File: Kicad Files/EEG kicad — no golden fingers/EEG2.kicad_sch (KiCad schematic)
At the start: 263 parts, among them J1 Conn_01x05_Pin, J2 Conn_01x11_Pin, U1 AD5293, U10 LF356N, U11 LF356N, U12 LF356N, U123 LF356N, U124 AD5293, U125 AD5293, U126 AD5293, U127 AD5293, U128 AD5293, U13 LF356N, U14 AD5293, U15 INA823, U16 INA823, U17 LF356N, U18 LF356N, U19 LF356N, U2 INA823, U20 LF356N, U21 LF356N, U22 LF356N, U23 LF356N, U24 LF356N, U25 AD5293, U26 AD5293, U27 INA823, U28 LF356N, U29 LF356N, U3 LF356N, U30 LF356N, U31 LF356N, U32 AD5293, U4 LF356N, U5 LF356N, U6 LF356N, U7 Teensy4.1, U75 INA823, U76 INA823, U77 INA823, U78 INA823, U79 INA823, U80 LF356N, U81 LF356N, U82 LF356N, U83 LF356N, U84 LF356N, U85 LF356N, U86 LF356N, U87 LF356N, U88 LF356N, U89 LF356N, U9 INA823, U90 LF356N, U91 LF356N, U92 LF356N, U93 LF356N, U94 LF356N, U95 LF356N, U96 LF356N, U97 LF356N, U98 LF356N

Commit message: Corrections in EEG
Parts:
- removed C101, C103, C104, C105, C106, C107, C108, C109, C11, C111, C112, C141, C142, C5: 0.22uF, Capacitor_SMD:C_0603_1608Metric, symbol Device:C
- removed C144, C145, C146, C147, C18, C20, C28, C45, C86, C87, C88, C89, C96, C97, C98, C99: 1uF, Capacitor_SMD:C_0805_2012Metric, symbol Device:C
- removed J2: Conn_01x11_Pin, Connector_PinHeader_1.27mm:PinHeader_1x11_P1.27mm_Vertical, symbol Connector:Conn_01x11_Pin
- removed R12, R249, R250, R251, R252: 150k, symbol Device:R
- removed R146, R147, R148, R149, R168, R170, R173, R176, R187, R188, R189, R190, R191, R192, R242, R243: 1k, symbol Device:R
- removed R15, R155, R157, R158, R159: 1326, symbol Device:R
- removed R151, R152, R154, R156, R161, R162, R163, R164, R31, R32: 2652, symbol Device:R
- removed R167, R169, R172, R175, R35, R5: 100, symbol Device:R
- removed R174, R177, R178, R179, R181, R182, R183, R184, R20, R244, R245, R246, R247, R40: 10k, symbol Device:R
- removed U1, U125, U126, U127, U128, U14, U25: AD5293, Package_SO:TSSOP-14_4.4x5mm_P0.65mm, symbol Potentiometer_Digital:AD5293
- removed U123, U20, U3, U4, U5, U82, U83, U84, U85, U86, U87, U88, U89, U91, U92, U93, U94, U96, U97, U98: LF356N, symbol Amplifier_Operational:LF357
- removed U15, U16, U76, U77, U78, U79, U9: INA823, Package_SO:VSSOP-8_3x3mm_P0.65mm, symbol Amplifier_Instrumentation:INA333xxDGK
- added C29, C31, C32, C33, C34, C49, C51, C52, C53, C54, C55, C56, C57, C59: 0.22uF, Capacitor_SMD:C_0603_1608Metric, symbol Device:C
- added C61, C62, C63, C64, C65, C66, C67, C69, C70, C72, C73, C74, C76, C77, C78, C79: 1uF, Capacitor_SMD:C_0805_2012Metric, symbol Device:C
- added J1: Conn_02x20_Top_Bottom, Connector_PinHeader_1.00mm:GoldFingers_1x40_0.155mm_DoubleSided, symbol Connector_Generic:Conn_02x20_Top_Bottom
- added R100, R103, R106, R108: 100, Resistor_SMD:R_0805_2012Metric, symbol Device:R
- added R101, R49, R52, R53, R54, R76, R77, R78, R79, R91, R92, R93, R94, R96, R97, R98: 10k, Resistor_SMD:R_0603_1608Metric, symbol Device:R
- added R102, R105, R107, R126, R127, R128, R129, R80, R81, R83, R84, R85, R86, R87, R88, R99: 1k, Resistor_SMD:R_0402_1005Metric, symbol Device:R
- added R111, R112, R113, R114, R119, R121, R123, R124: 2.64k, Resistor_SMD:R_0603_1608Metric, symbol Device:R
- added R116, R117, R118, R120: 1.32k, Resistor_SMD:R_0805_2012Metric, symbol Device:R
- added R56, R57, R58, R59, R60, R61, R62, R63, R64, R66, R67, R68, R69, R71, R72, R73, R74, R75: 150k, Resistor_SMD:R_0402_1005Metric, symbol Device:R
- added U1, U3, U4, U57, U58, U59, U60: INA823, Package_SO:VSSOP-8_3x3mm_P0.65mm, symbol Amplifier_Instrumentation:INA333xxDGK
- added U16, U37, U38, U39, U40, U42, U43, U44, U45, U47, U48, U49, U50, U51, U52, U53, U54, U7, U8, U9: LF356M, LF356M:SOIC127P599X175-8N, symbol Amplifier_Operational:LF357
- added U27, U28, U29, U32, U33, U34, U35: AD5293, AD5293:AD5293, symbol Potentiometer_Digital:AD5293
- C12, C13, C4, C6: value 0.22uF -> 1uF; footprint Capacitor_SMD:C_0603_1608Metric -> Capacitor_SMD:C_0805_2012Metric
- C27, C46, C47, C48: value 1uF -> 0.22uF; footprint Capacitor_SMD:C_0805_2012Metric -> Capacitor_SMD:C_0603_1608Metric
- R1, R22, R26, R41, R42, R43, R44: footprint (none) -> Resistor_SMD:R_0402_1005Metric
- R10, R18, R6: value 1k -> 2.64k; footprint (none) -> Resistor_SMD:R_0603_1608Metric
- R104: renamed from R171; footprint (none) -> Resistor_SMD:R_0603_1608Metric
- R109: renamed from R166; footprint (none) -> Resistor_SMD:R_0402_1005Metric
- R11: value 10k -> 1.32k; footprint (none) -> Resistor_SMD:R_0805_2012Metric
- R110: renamed from R165; footprint (none) -> Resistor_SMD:R_0805_2012Metric
- R115: renamed from R160; value 2652 -> 2.64k; footprint (none) -> Resistor_SMD:R_0603_1608Metric
- R12: renamed from R50; value 2652 -> 2.64k; footprint (none) -> Resistor_SMD:R_0603_1608Metric
- R122: renamed from R153; value 1326 -> 1.32k; footprint (none) -> Resistor_SMD:R_0805_2012Metric
- R125: renamed from R150; value 2652 -> 2.64k; footprint (none) -> Resistor_SMD:R_0603_1608Metric
- R13, R9: value 1k -> 1.32k; footprint (none) -> Resistor_SMD:R_0805_2012Metric
- R130: renamed from R145; footprint (none) -> Resistor_SMD:R_0402_1005Metric
- R14: value 2652 -> 1.32k; footprint (none) -> Resistor_SMD:R_0805_2012Metric
- R15: renamed from R51; value 1326 -> 1.32k; footprint (none) -> Resistor_SMD:R_0805_2012Metric
- R16: value 2652 -> 2.64k; footprint (none) -> Resistor_SMD:R_0603_1608Metric
- R17: value 100 -> 2.64k; footprint (none) -> Resistor_SMD:R_0603_1608Metric
- R19, R7, R8: value 10k -> 2.64k; footprint (none) -> Resistor_SMD:R_0603_1608Metric
- R2, R4: value 2652 -> 1k; footprint (none) -> Resistor_SMD:R_0402_1005Metric
- R20: renamed from R52; value 2652 -> 2.64k; footprint (none) -> Resistor_SMD:R_0603_1608Metric
- R21, R25: value 1k -> 100; footprint (none) -> Resistor_SMD:R_0805_2012Metric
- R23: value 10k -> 100; footprint (none) -> Resistor_SMD:R_0805_2012Metric
- R24, R47, R48: value 150k -> 1k; footprint (none) -> Resistor_SMD:R_0402_1005Metric
- R27: value 2652 -> 10k; footprint (none) -> Resistor_SMD:R_0603_1608Metric
- R28: value 2652 -> 100; footprint (none) -> Resistor_SMD:R_0805_2012Metric
- R29, R3: value 1326 -> 1k; footprint (none) -> Resistor_SMD:R_0402_1005Metric
- R30: value 1326 -> 10k; footprint (none) -> Resistor_SMD:R_0603_1608Metric
- R31: renamed from R53; footprint (none) -> Resistor_SMD:R_0805_2012Metric
- R32: renamed from R54; footprint (none) -> Resistor_SMD:R_0402_1005Metric
- R33: value 100 -> 10k; footprint (none) -> Resistor_SMD:R_0603_1608Metric
- R34, R36: value 1k -> 10k; footprint (none) -> Resistor_SMD:R_0603_1608Metric
- R35: renamed from R55; footprint (none) -> Resistor_SMD:R_0603_1608Metric
- R37, R38, R39: footprint (none) -> Resistor_SMD:R_0603_1608Metric
- R40: renamed from R56; footprint (none) -> Resistor_SMD:R_0603_1608Metric
- R45, R46: value 10k -> 1k; footprint (none) -> Resistor_SMD:R_0402_1005Metric
- R5: renamed from R49; footprint (none) -> Resistor_SMD:R_0402_1005Metric
- R50: renamed from R57; footprint (none) -> Resistor_SMD:R_0402_1005Metric
- R51: renamed from R58; footprint (none) -> Resistor_SMD:R_0402_1005Metric
- R55: renamed from R59; footprint (none) -> Resistor_SMD:R_0603_1608Metric
- R65: renamed from R60; footprint (none) -> Resistor_SMD:R_0402_1005Metric
- R70: renamed from R248; footprint (none) -> Resistor_SMD:R_0402_1005Metric
- R82: renamed from R241; footprint (none) -> Resistor_SMD:R_0603_1608Metric
- R89: renamed from R186; footprint (none) -> Resistor_SMD:R_0402_1005Metric
- R90: renamed from R185; footprint (none) -> Resistor_SMD:R_0402_1005Metric
- R95: renamed from R180; footprint (none) -> Resistor_SMD:R_0603_1608Metric
- U10, U11, U12, U13, U17, U18, U19, U21, U22, U23, U24, U6: value LF356N -> LF356M; footprint (none) -> LF356M:SOIC127P599X175-8N
- U14: renamed from U28; value LF356N -> LF356M; footprint (none) -> LF356M:SOIC127P599X175-8N
- U15: renamed from U29; value LF356N -> LF356M; footprint (none) -> LF356M:SOIC127P599X175-8N
- U20: renamed from U30; value LF356N -> LF356M; footprint (none) -> LF356M:SOIC127P599X175-8N
- U25: renamed from U31; value LF356N -> LF356M; footprint (none) -> LF356M:SOIC127P599X175-8N
- U26: footprint Package_SO:TSSOP-14_4.4x5mm_P0.65mm -> AD5293:AD5293
- U30: renamed from U32; footprint Package_SO:TSSOP-14_4.4x5mm_P0.65mm -> AD5293:AD5293
- U36: renamed from U124; footprint Package_SO:TSSOP-14_4.4x5mm_P0.65mm -> AD5293:AD5293
- U41: renamed from U95; value LF356N -> LF356M; footprint (none) -> LF356M:SOIC127P599X175-8N
- U46: renamed from U90; value LF356N -> LF356M; footprint (none) -> LF356M:SOIC127P599X175-8N
- U55: renamed from U81; value LF356N -> LF356M; footprint (none) -> LF356M:SOIC127P599X175-8N
- U56: renamed from U80; value LF356N -> LF356M; footprint (none) -> LF356M:SOIC127P599X175-8N
- renumbered C30 to C11, C40 to C18, C31 to C20, C32 to C28, C33 to C30, C34 to C35, C35 to C40, C143 to C45, C29 to C5, C110 to C50, C102 to C58, C100 to C60, C94 to C68, C49 to C71, C50 to C75, C85 to C80, J1 to J2, U7 to U31, U27 to U5, U75 to U61
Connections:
- net Electrode1: now also J1.1 (Pin_1), U1.3 (+); no longer U2.3 (+)
- net Electrode10: now also J1.20 (Pin_20)
- net Electrode2: now also U2.3 (+), J1.3 (Pin_3)
- net Electrode3: now also J1.5 (Pin_5), U3.3 (+)
- net Electrode4: now also J1.7 (Pin_7), U4.3 (+)
- net Electrode5: now also J1.9 (Pin_9)
- net Electrode6: now also J1.12 (Pin_12), U57.3 (+)
- net Electrode7: now also J1.14 (Pin_14), U58.3 (+)
- net Electrode8: now also J1.16 (Pin_16), U59.3 (+)
- net Electrode9: now also J1.18 (Pin_18), U60.3 (+)
- net GND: now also C24.2, C46.2, C47.2, C48.2, R26.2, R29.2, R46.2, C31.2, C32.2, C33.2, C34.2, C49.2, C53.2, C55.2, C57.2, C59.2, R102.2, R105.2, R107.2, R61.2, R62.2, R63.2, R64.2, R66.2, R67.2, R68.2, R69.2, R80.2, R83.2, R85.2, R87.2, R99.2, U1.4 (V-), U1.5 (Ref), U16.4 (V-), U27.2 (Vss-), U27.5 (RL), U27.9 (GND), U28.2 (Vss-), U28.5 (RL), U28.9 (GND), U29.2 (Vss-), U29.5 (RL), U29.9 (GND), U3.4 (V-), U3.5 (Ref), U32.2 (Vss-), U32.5 (RL), U32.9 (GND), U33.2 (Vss-), U33.5 (RL), U33.9 (GND), U34.2 (Vss-), U34.5 (RL), U34.9 (GND), U35.2 (Vss-), U35.5 (RL), U35.9 (GND), U37.4 (V-), U38.4 (V-), U39.4 (V-), U4.4 (V-), U4.5 (Ref), U40.4 (V-), U42.4 (V-), U43.4 (V-), U44.4 (V-), U45.4 (V-), U47.4 (V-), U48.4 (V-), U49.4 (V-), U50.4 (V-), U51.4 (V-), U52.4 (V-), U53.4 (V-), U54.4 (V-), U57.4 (V-), U57.5 (Ref), U58.4 (V-), U58.5 (Ref), U59.4 (V-), U59.5 (Ref), U60.4 (V-), U60.5 (Ref), U7.4 (V-), U8.4 (V-), U9.4 (V-); no longer C13.2, C25.2, C4.2, C6.2, R10.2, R18.2, R34.2, R36.2, R47.2, R6.2
- net Ref_Electrode: now also J1.30 (Pin_30), U1.2 (-), U3.2 (-), U4.2 (-), U57.2 (-), U58.2 (-), U59.2 (-), U60.2 (-)
- net Vss: now also U1.7 (V+), U16.7 (V+), U27.6 (Vdd+), U27.8 (Vlog), U28.6 (Vdd+), U28.8 (Vlog), U29.6 (Vdd+), U29.8 (Vlog), U3.7 (V+), U32.6 (Vdd+), U32.8 (Vlog), U33.6 (Vdd+), U33.8 (Vlog), U34.6 (Vdd+), U34.8 (Vlog), U35.6 (Vdd+), U35.8 (Vlog), U37.7 (V+), U38.7 (V+), U39.7 (V+), U4.7 (V+), U40.7 (V+), U42.7 (V+), U43.7 (V+), U44.7 (V+), U45.7 (V+), U47.7 (V+), U48.7 (V+), U49.7 (V+), U50.7 (V+), U51.7 (V+), U52.7 (V+), U53.7 (V+), U54.7 (V+), U57.7 (V+), U58.7 (V+), U59.7 (V+), U60.7 (V+), U7.7 (V+), U8.7 (V+), U9.7 (V+)
- net at C41.1: now also R71.2, U37.6; no longer C42.1
- net at U11.2 (-), U11.6: now also R25.1, R33.1; no longer R17.1, R19.1
- net Electrode Output 5: now reaches U31.40 (18_A4_SDA)
- net Electrode Output 5: now also C40.2, R65.1
- net Electrode Output 8: now reaches C43.2
- net Electrode Output 8: now also U31.43 (21_A7_RX5_BCLK1), R68.1; no longer C44.2
- net at C44.1: now also R74.2, U40.6; no longer C43.1
- net at C8.2: now also C14.2, R18.2, R8.1; no longer C10.1
- net at U10.2 (-), U10.6: now also C14.1, C8.1, R13.2; no longer C37.1, C9.1
- net SDI: now reaches U26.10 (SDI), U30.10 (SDI), U31.13 (11_MOSI_CTX1), U36.10 (SDI)
- net SDI: now also U27.10 (SDI), U28.10 (SDI), U29.10 (SDI), U32.10 (SDI), U33.10 (SDI), U34.10 (SDI), U35.10 (SDI)
- net CLK: now reaches U26.11 (CLK), U30.11 (CLK), U31.35 (13_SCK_LED), U36.11 (CLK)
- net CLK: now also U27.11 (CLK), U28.11 (CLK), U29.11 (CLK), U32.11 (CLK), U33.11 (CLK), U34.11 (CLK), U35.11 (CLK)
- net CS 1: now reaches U26.12 (~{CS})
- net CS 1: now also U31.14 (12_MISO_MQSL); no longer U31.7 (5_IN2)
- net at U26.3 (RH): now also U21.2 (-); no longer U24.2 (-)
- net at U24.6: now also C39.1, R59.2; no longer U26.4 (RW)
- net at R9.1: now also C1.2, C13.1; no longer R11.1
- net at R7.2: now also C2.1, U2.6; no longer R8.1
- net at R13.1: now also C17.1, C3.2
- net at R14.2: now also C16.1, C9.1, U12.2 (-), U12.6; no longer C8.1
- net at R30.1: now also R23.1, U9.2 (-), U9.6; no longer C16.2
- net at R27.2: now also C23.2, R36.1; no longer C15.1
- net at R25.2: now also R26.1, U10.3 (+)
- net at R7.1: now also C12.2, C7.2, R17.2
- net at R4.1: now also U4.1 (Rg); no longer C3.2
- net at R21.2, R22.1: now also U6.3 (+); no longer U12.2 (-)
- net at U12.3 (+): now also R28.2, R29.1
- net at U18.3 (+): now also C24.1, R38.2; no longer C19.2
- net at C45.1, U41.6: now also R75.2; no longer U36.4 (RW)
- net at R6.1: now also C10.2, C6.2, R16.2
- net at U23.2 (-): now also U28.3 (RH)
- net at U23.6: now also C38.1, R58.2; no longer C27.1
- net at C23.1, R41.1: now also R49.1, U16.6; no longer R45.1, U21.6
- net at C40.1, U25.6: now also R60.2; no longer U30.4 (RW)
- net Electrode Output 6: now reaches C41.2
- net Electrode Output 6: now also U31.41 (19_A5_SCL), R66.1; no longer C42.2
- net CS 10: now reaches U36.12 (~{CS})
- net CS 10: now also U31.4 (2_OUT2); no longer U31.9 (7_RX2_OUT1A)
- net at R41.2, R42.1: now also U16.2 (-); no longer U21.2 (-)
- net CS 9: now reaches U31.5 (3_LRCLK2)
- net CS 9: now also U35.12 (~{CS})
- net at U13.2 (-): now also R28.1, R34.1, U13.6
- net at R19.2: now also C16.2, C9.2, R10.1; no longer C12.2
- net at R9.2: now also C10.1, C6.1, U6.2 (-), U6.6; no longer R10.1
- net at R8.2: now also C3.1, U3.6; no longer C4.1
- net Electrode Output 4: now reaches C39.2
- net Electrode Output 4: now also U31.39 (17_A3_TX4_SDA1), R64.1; no longer R28.1
- net at R48.1: now also R47.2, U19.2 (-); no longer U31.44 (22_A8_CTX1)
- net at C48.1: now also R78.2, U39.3 (+); no longer C47.1
- net at C46.1: now also R76.2, U37.3 (+)
- net CS 2: now reaches U31.12 (10_CS_MQSR)
- net CS 2: now also U27.12 (~{CS})
- net Electrode Output 3: now reaches U31.38 (16_A2_RX4_SCL1)
- net Electrode Output 3: now also C38.2, R63.1
- net CS 5: now reaches U30.12 (~{CS})
- net CS 5: now also U31.9 (7_RX2_OUT1A); no longer U31.8 (6_OUT1D)
- net at R38.1: now also C27.2, R33.2
- net at R43.2, R44.1: now also U17.2 (-); no longer U22.2 (-)
- net at C22.1: now also R37.2, U17.3 (+); no longer U22.3 (+)
- net Electrode Output 2: now reaches U31.37 (15_A1_RX3_SPDIF_IN)
- net Electrode Output 2: now also C37.2, R62.1
- net Electrode Output 10: now reaches C45.2, R70.1
- net Electrode Output 10: now also U31.45 (23_A9_CRX1_MCLK1); no longer U31.36 (14_A0_TX3_SPDIF_OUT)
- net at R1.1: now also U1.1 (Rg); no longer U2.1 (Rg)
- net at R1.2: now also U1.8 (Rg); no longer U2.8 (Rg)
- net CS 8: now reaches U31.6 (4_BCLK2)
- net CS 8: now also U34.12 (~{CS})
- net at U19.3 (+): now also C26.1, R39.2; no longer R36.1
- net at C7.1: now also C12.1, R11.2, U8.2 (-), U8.6; no longer U6.6
- net CS 4: now reaches U31.10 (8_TX2_IN1)
- net CS 4: now also U29.12 (~{CS})
- net CS 3: now reaches U31.11 (9_OUT1C)
- net CS 3: now also U28.12 (~{CS})
- new net: U32.3 (RH), U37.2 (-)
- new net: R71.1, U32.4 (RW)
- new net: C62.1, C77.2, R117.1
- new net: C62.2, R112.1, U49.3 (+)
- new net: C67.1, C73.1, R113.2, R123.1
- new net: C78.1, R123.2, U59.6
- new net: C1.1, R6.2, U1.6
- new net: C51.1, R76.1, R81.1, U42.6
- new net: C51.2, R91.1, R96.2
- new net: C33.1, R53.2, U23.3 (+)
- new net: R103.1, R97.1, U49.2 (-), U49.6
- new net: C52.2, R92.1, R97.2
- new net: C29.1, R47.1, R54.1, U19.6
- new net: C34.1, R54.2, U24.3 (+)
- new net: C55.1, R92.2, U43.3 (+)
- new net: C17.2, R18.1, U11.3 (+)
- new net: R128.1, U59.1 (Rg)
- new net: R128.2, U59.8 (Rg)
- new net: C29.2, R34.2, R39.1
- new net: R21.1, R27.1, U7.2 (-), U7.6
- new net: C53.1, R91.2, U42.3 (+)
- new net: C77.1, R121.2, U58.6
- new net: R126.1, U57.1 (Rg)
- new net: R126.2, U57.8 (Rg)
- new net: R3.1, U3.1 (Rg)
- new net: R3.2, U3.8 (Rg)
- new net: R4.2, U4.8 (Rg)
- new net: R100.1, R96.1, U47.2 (-), U47.6
- new net: R100.2, R99.1, U48.3 (+)
- new net: R80.1, R81.2, U42.2 (-)
- new net: C25.2, R30.2, R37.1
- new net: C25.1, R43.1, R52.1, U17.6
- new net: C21.1, R36.2, U16.3 (+)
- new net: C32.1, R52.2, U22.3 (+)
- new net: C76.1, R119.2, U57.6
- new net: C61.1, C76.2, R116.1
- new net: C15.1, C2.2, R11.1
- new net: R75.1, U36.4 (RW)
- new net: R23.2, R24.1, U8.3 (+)
- new net: U35.3 (RH), U40.2 (-)
- new net: R74.1, U35.4 (RW)
- new net: C56.1, R79.1, R88.1, U45.6
- new net: C56.2, R101.2, R94.1
- new net: C36.1, R56.2, U21.6
- new net: C64.1, C78.2, R118.1
- new net: C67.2, C73.2, R118.2, U52.2 (-), U52.6
- new net: R72.1, U33.4 (RW)
- new net: C42.1, R72.2, U38.6
- new net: R105.1, R106.2, U52.3 (+)
- new net: C66.1, C79.2, R120.1
- new net: C69.2, C74.2, R120.2, U54.2 (-), U54.6
- new net: R56.1, U26.4 (RW)
- new net: R58.1, U28.4 (RW)
- new net: R59.1, U29.4 (RW)
- new net: R87.1, R88.2, U45.2 (-)
- new net: C65.1, C72.1, R112.2, R121.1
- new net: C65.2, C72.2, R117.2, U50.2 (-), U50.6
- new net: R45.2, R46.1, U18.2 (-)
- new net: C27.1, R45.1, R53.1, U18.6
- new net: R60.1, U30.4 (RW)
- new net: R106.1, R98.1, U51.2 (-), U51.6
- new net: R83.1, R84.2, U43.2 (-)
- new net: C52.1, R77.1, R84.1, U43.6
- new net: C64.2, R113.1, U51.3 (+)
- new net: C63.1, C70.1, R111.2, R119.1
- new net: C63.2, C70.2, R116.2, U48.2 (-), U48.6
- new net: U22.2 (-), U27.3 (RH)
- new net: C37.1, R57.2, U22.6
- new net: C54.1, R78.1, R86.1, U44.6
- new net: C31.1, R49.2, U21.3 (+)
- new net: C61.2, R111.1, U47.3 (+)
- new net: R101.1, R108.1, U53.2 (-), U53.6
- new net: R107.1, R108.2, U54.3 (+)
- new net: R57.1, U27.4 (RW)
- new net: C57.1, R93.2, U44.3 (+)
- new net: C19.1, C4.2, R14.1
- new net: C19.2, R19.1, U13.3 (+)
- new net: C15.2, R17.1, U9.3 (+)
- new net: C49.1, R79.2, U40.3 (+)
- new net: C59.1, R94.2, U45.3 (+)
- new net: R127.1, U58.1 (Rg)
- new net: R127.2, U58.8 (Rg)
- new net: R102.1, R103.2, U50.3 (+)
- new net: R129.1, U60.1 (Rg)
- new net: C79.1, R124.2, U60.6
- new net: R129.2, U60.8 (Rg)
- new net: C69.1, C74.1, R114.2, R124.1
- new net: C66.2, R114.1, U53.3 (+)
- new net: R85.1, R86.2, U44.2 (-)
- new net: C47.1, R77.2, U38.3 (+)
- new net: R2.1, U2.1 (Rg)
- new net: R2.2, U2.8 (Rg)
- new net: C4.1, R10.2, U4.6
- new net: U34.3 (RH), U39.2 (-)
- new net: C43.1, R73.2, U39.6
- new net: C13.2, R16.1, U7.3 (+)
- new net: R73.1, U34.4 (RW)
- new net: U24.2 (-), U29.3 (RH)
- new net: C54.2, R93.1, R98.2
- new net: U33.3 (RH), U38.2 (-)
- new net CS 6: U31.8 (6_OUT1D), U32.12 (~{CS})
- new net CS 7: U31.7 (5_IN2), U33.12 (~{CS})
- new net Electrode Output 1: C36.2, R61.1, U31.36 (14_A0_TX3_SPDIF_OUT)
- new net Electrode Output 7: C42.2, R67.1, U31.42 (20_A6_TX5_LRCLK1)
- new net Electrode Output 9: C44.2, R69.1, U31.44 (22_A8_CTX1)
- no-connect marks 144 -> 173
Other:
- moved on the sheet: C11, C18, C20, C28, C30, C35, C40, C45, C5, C50, C58, C60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

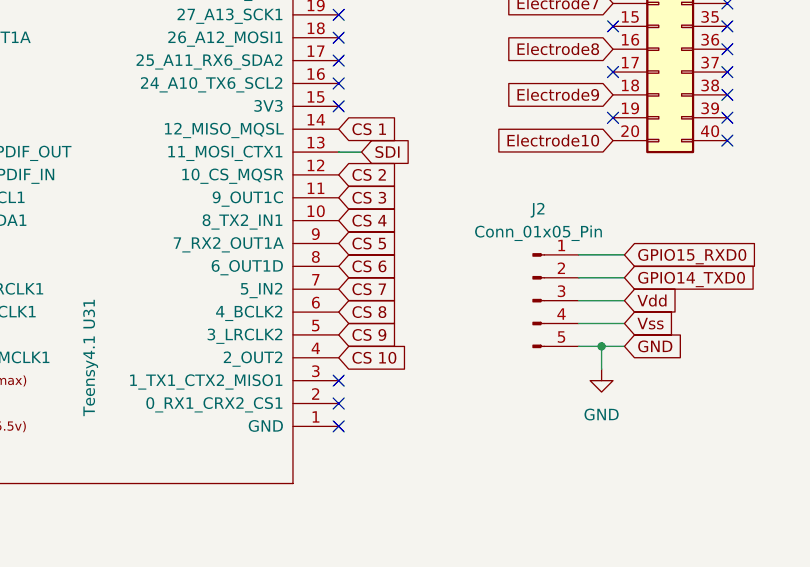
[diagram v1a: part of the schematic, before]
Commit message: Working on EEG
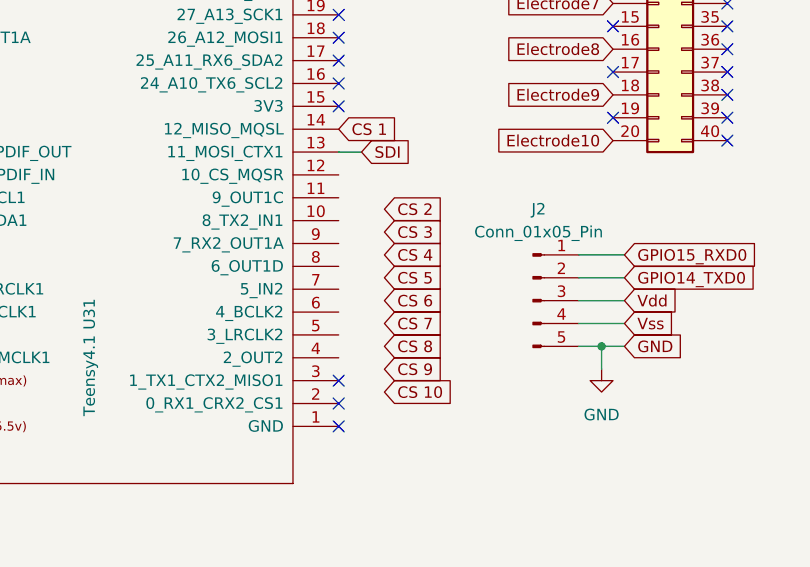
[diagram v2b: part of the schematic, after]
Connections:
- net CS 10: no longer U31.4 (2_OUT2)
- net CS 2: no longer U31.12 (10_CS_MQSR)
- net CS 3: no longer U31.11 (9_OUT1C)
- net CS 4: no longer U31.10 (8_TX2_IN1)
- net CS 5: no longer U31.9 (7_RX2_OUT1A)
- net CS 6: no longer U31.8 (6_OUT1D)
- net CS 7: no longer U31.7 (5_IN2)
- net CS 8: no longer U31.6 (4_BCLK2)
- net CS 9: no longer U31.5 (3_LRCLK2)
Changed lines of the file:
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@@
 	(global_label "CS 10"
 		(shape input)
-		(at 292.1 93.98 0)
-		(fields_autoplaced yes)
-		(effects
-			(font
-				(size 1.27 1.27)
-			)
-			(justify left)
-		)
-		(property "Intersheetrefs" "${INTERSHEET_REFS}"
-			(at 300.9513 93.98 0)
+		(at 297.18 97.79 0)
+		(fields_autoplaced yes)
+		(effects
+			(font
+				(size 1.27 1.27)
+			)
+			(justify left)
+		)
+		(property "Intersheetrefs" "${INTERSHEET_REFS}"
+			(at 306.0313 97.79 0)
 			(effects
 				(font
@@
 	(global_label "CS 9"
 		(shape input)
-		(at 292.1 91.44 0)
-		(fields_autoplaced yes)
-		(effects
-			(font
-				(size 1.27 1.27)
-			)
-			(justify left)
-		)
-		(property "Intersheetrefs" "${INTERSHEET_REFS}"
-			(at 299.7418 91.44 0)
+		(at 297.18 95.25 0)
+		(fields_autoplaced yes)
+		(effects
+			(font
+				(size 1.27 1.27)
+			)
+			(justify left)
+		)
+		(property "Intersheetrefs" "${INTERSHEET_REFS}"
+			(at 304.8218 95.25 0)
 			(effects
 				(font
@@
 	(global_label "CS 4"
 		(shape input)
-		(at 292.1 78.74 0)
-		(fields_autoplaced yes)
-		(effects
-			(font
-				(size 1.27 1.27)
-			)
-			(justify left)
-		)
-		(property "Intersheetrefs" "${INTERSHEET_REFS}"
-			(at 299.7418 78.74 0)
+		(at 297.18 82.55 0)
+		(fields_autoplaced yes)
+		(effects
+			(font
+				(size 1.27 1.27)
+			)
+			(justify left)
+		)
+		(property "Intersheetrefs" "${INTERSHEET_REFS}"
+			(at 304.8218 82.55 0)
 			(effects
 				(font
@@
 	(global_label "CS 2"
 		(shape input)
-		(at 292.1 73.66 0)
-		(fields_autoplaced yes)
-		(effects
-			(font
-				(size 1.27 1.27)
-			)
-			(justify left)
-		)
-		(property "Intersheetrefs" "${INTERSHEET_REFS}"
-			(at 299.7418 73.66 0)
+		(at 297.18 77.47 0)
+		(fields_autoplaced yes)
+		(effects
+			(font
+				(size 1.27 1.27)
+			)
+			(justify left)
+		)
+		(property "Intersheetrefs" "${INTERSHEET_REFS}"
+			(at 304.8218 77.47 0)
 			(effects
 				(font
@@
 	(global_label "CS 5"
 		(shape input)
-		(at 292.1 81.28 0)
-		(fields_autoplaced yes)
-		(effects
-			(font
-				(size 1.27 1.27)
-			)
-			(justify left)
-		)
-		(property "Intersheetrefs" "${INTERSHEET_REFS}"
-			(at 299.7418 81.28 0)
+		(at 297.18 85.09 0)
+		(fields_autoplaced yes)
+		(effects
+			(font
+				(size 1.27 1.27)
+			)
+			(justify left)
+		)
+		(property "Intersheetrefs" "${INTERSHEET_REFS}"
+			(at 304.8218 85.09 0)
 			(effects
 				(font
@@
 	(global_label "CS 3"
 		(shape input)
-		(at 292.1 76.2 0)
-		(fields_autoplaced yes)
-		(effects
-			(font
-				(size 1.27 1.27)
-			)
-			(justify left)
-		)
-		(property "Intersheetrefs" "${INTERSHEET_REFS}"
-			(at 299.7418 76.2 0)
+		(at 297.18 80.01 0)
+		(fields_autoplaced yes)
+		(effects
+			(font
+				(size 1.27 1.27)
+			)
+			(justify left)
+		)
+		(property "Intersheetrefs" "${INTERSHEET_REFS}"
+			(at 304.8218 80.01 0)
 			(effects
 				(font
@@
 	(global_label "CS 6"
 		(shape input)
-		(at 292.1 83.82 0)
-		(fields_autoplaced yes)
-		(effects
-			(font
-				(size 1.27 1.27)
-			)
-			(justify left)
-		)
-		(property "Intersheetrefs" "${INTERSHEET_REFS}"
-			(at 299.7418 83.82 0)
+		(at 297.18 87.63 0)
+		(fields_autoplaced yes)
+		(effects
+			(font
+				(size 1.27 1.27)
+			)
+			(justify left)
+		)
+		(property "Intersheetrefs" "${INTERSHEET_REFS}"
+			(at 304.8218 87.63 0)
 			(effects
 				(font
@@
 	(global_label "CS 7"
 		(shape input)
-		(at 292.1 86.36 0)
-		(fields_autoplaced yes)
-		(effects
-			(font
-				(size 1.27 1.27)
-			)
-			(justify left)
-		)
-		(property "Intersheetrefs" "${INTERSHEET_REFS}"
-			(at 299.7418 86.36 0)
+		(at 297.18 90.17 0)
+		(fields_autoplaced yes)
+		(effects
+			(font
+				(size 1.27 1.27)
+			)
+			(justify left)
+		)
+		(property "Intersheetrefs" "${INTERSHEET_REFS}"
+			(at 304.8218 90.17 0)
 			(effects
 				(font
@@
 	(global_label "CS 8"
 		(shape input)
-		(at 292.1 88.9 0)
-		(fields_autoplaced yes)
-		(effects
-			(font
-				(size 1.27 1.27)
-			)
-			(justify left)
-		)
-		(property "Intersheetrefs" "${INTERSHEET_REFS}"
-			(at 299.7418 88.9 0)
-			(effects
-				(font
+		(at 297.18 92.71 0)
+		(fields_autoplaced yes)
+		(effects
+			(font
+				(size 1.27 1.27)
+			)
+			(justify left)
+		)
+		(property "Intersheetrefs" "${INTERSHEET_REFS}"
+			(at 304.8218 92.71 0)
+			(effects
+				(font
